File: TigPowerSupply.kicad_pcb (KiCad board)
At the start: 2 copper layers, 86.4 x 34.3 mm, 10 parts, among them J1 Screw_Terminal_01x02, J2 Conn_01x03, U1 MCP1826S

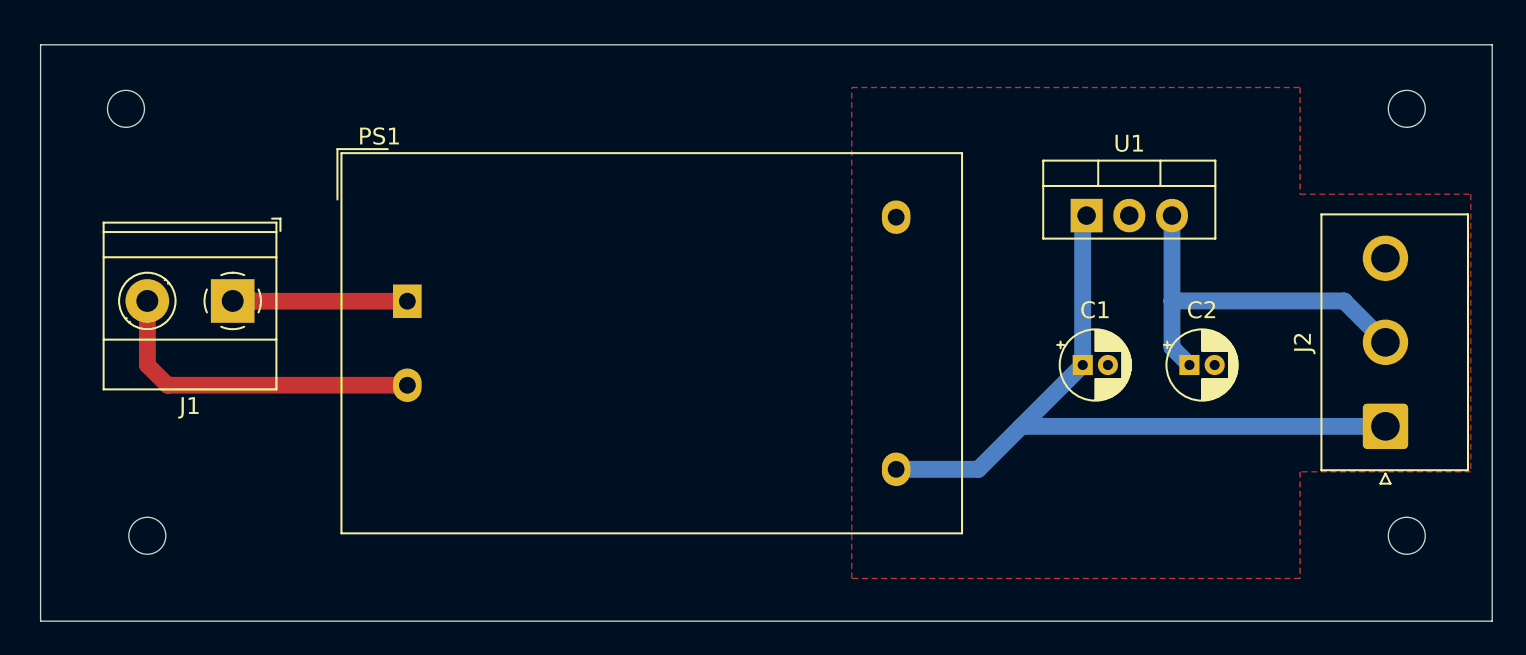
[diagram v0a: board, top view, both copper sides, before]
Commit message: tweaked the dimensions to be round mm values
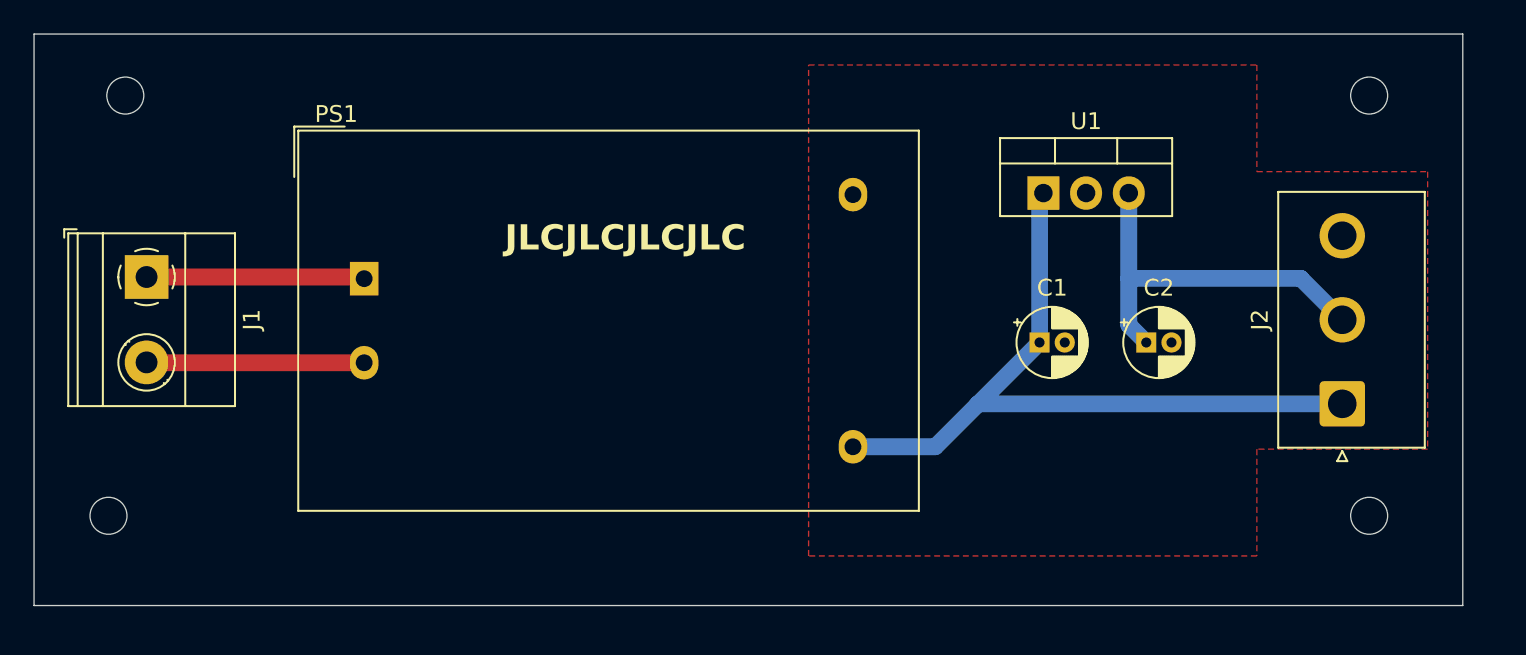
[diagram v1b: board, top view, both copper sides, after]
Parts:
- moved J1 5.32 mm to (78.7, 54.5), turned to -90 degrees
- moved C2 2.90 mm to (138.2, 58.4)
- moved PS1 2.90 mm to (91.6, 54.6)
- moved J2 2.90 mm to (149.8, 62.0)
- moved C1 2.90 mm to (131.8, 58.4)
- moved U1 2.90 mm to (132.1, 49.5)
- moved H2 2.60 mm to (76.4, 68.7)
- moved H4 2.54 mm to (151.4, 68.7)
- moved H3 2.38 mm to (151.4, 43.7)
- moved H1 0.79 mm to (77.4, 43.7)
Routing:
- net Net-(J1-Pin_2): track 19.8 -> 13.0 mm
- net Net-(J1-Pin_1): track 10.4 -> 13.0 mm
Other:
- board size 86.4 x 34.3 mm -> 85 x 34 mm
- board text added: "JLCJLCJLCJLC"
